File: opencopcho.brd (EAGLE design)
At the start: 51 parts, among them CON12 CON-4P-JST_GH-RA, CON13 CON-4P-JST_GH-RA, CON14 PINHEAD_1X02-2.54, CON15 PINHEAD_1X05-2.54-KEY, CON16 PINHEAD_1X05-2.54-KEY, CON17 PINHEAD_1X05-2.54-KEY, CON18 PINHEAD_1X05-2.54-KEY, CON5 CON-4P-JST_GH-RA, CON6 CON-4P-JST_GH-RA, CON7 PINHEAD_1X02-2.54, CON8 PINHEAD_2X04-PLS, CON9 PINHEAD_2X04-PLS, IC1 TPS54260, IC2 MCP2542WFD, IC6 MCP2542WFD

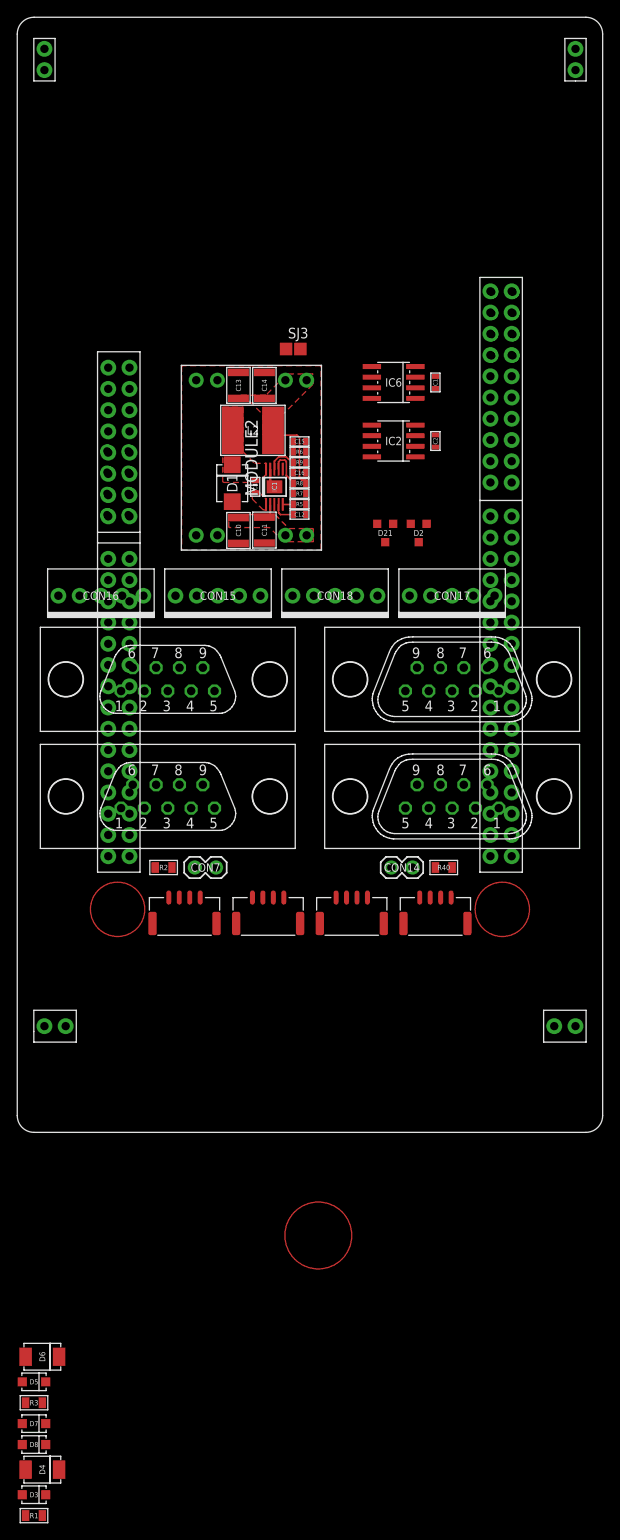
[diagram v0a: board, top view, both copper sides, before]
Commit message: updates
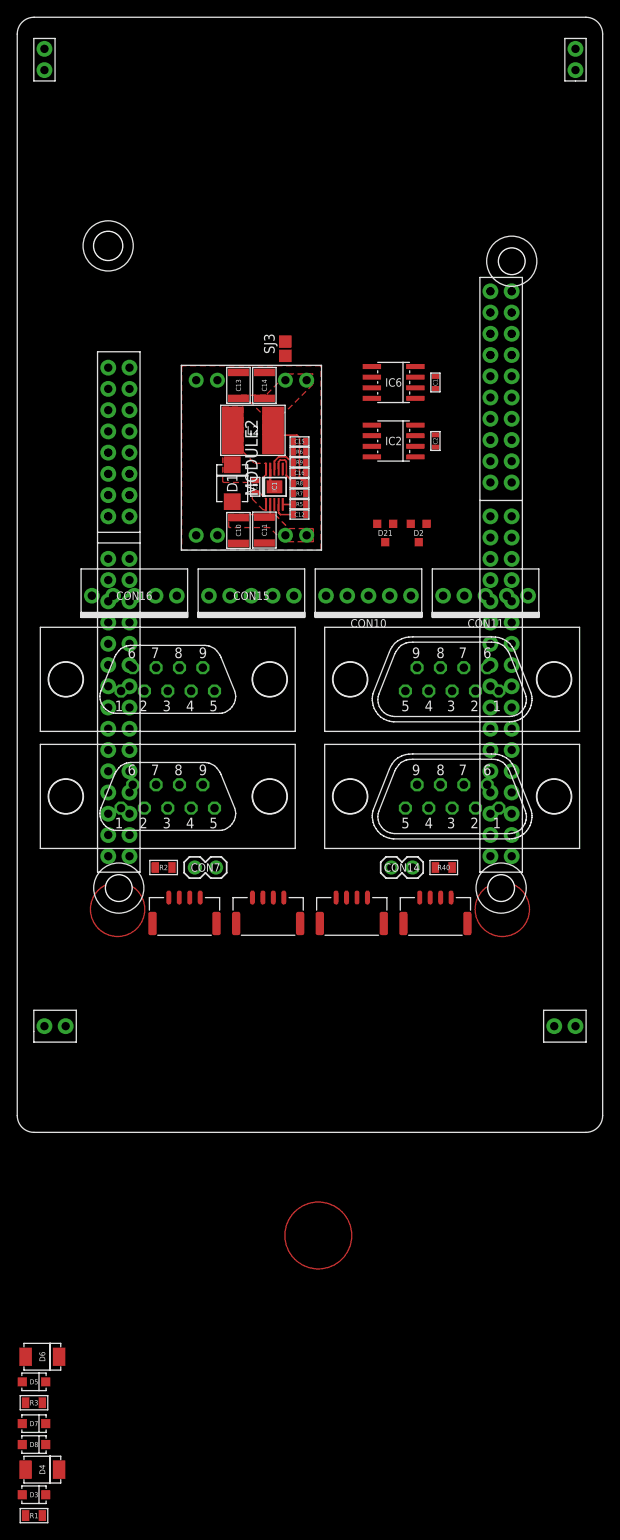
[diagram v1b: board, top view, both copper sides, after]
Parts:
- removed CON17, CON18: PINHEAD_1X05-2.54-KEY, pinhead:1X05-PTH-2.54-KEY
- added CON10, CON11: PINHEAD_1X05-2.54-KEY, pinhead:1X05-PTH-2.54-KEY
- moved CON15 4.00 mm to (-7.00, -2.50)
- moved CON16 4.00 mm to (-21.0, -2.50)
- moved SJ3 0.95 mm to (-2.95, 27.0), turned to 90 degrees
- moved CON9 0.25 mm to (-22.9, 10.8)
- moved CON8 0.17 mm to (22.9, 30.1)
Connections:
- net N$2 renamed VDD_24V
- removed net CAN_H: CON12.2, CON13.2, CON5.2, CON6.2, D2.1, D21.1, IC2.7, IC6.7, R2.1, R40.1
- removed net CAN_L: CON12.3, CON13.3, CON14.1, CON5.3, CON6.3, CON7.1, D2.2, D21.2, IC2.6, IC6.6
- new net CAN1_H: CON1.7, CON15.4, CON16.4, CON2.7, CON5.2, CON6.2, D2.1, IC2.7, R2.1
- new net CAN1_L: CON1.2, CON15.3, CON16.3, CON2.2, CON5.3, CON6.3, CON7.1, D2.2, IC2.6
- new net CAN1_SHIELD: CON15.2, CON16.2, CON2.5
- new net CAN1_VDD: CON1.9, CON15.5, CON16.5, CON2.9, R3.2
- new net CAN2_H: CON10.4, CON11.4, CON12.2, CON13.2, CON3.7, CON4.7, D21.1, IC6.7, R40.1
- new net CAN2_L: CON10.3, CON11.3, CON12.3, CON13.3, CON14.1, CON3.2, CON4.2, D21.2, IC6.6
- new net CAN2_SHIELD: CON10.2, CON11.2, CON3.5
- new net CAN2_VDD: CON10.5, CON11.5, CON3.9, R1.2
- net GND: now also CON1.6, CON10.1, CON11.1, CON15.1, CON16.1, CON2.6, CON3.6, CON4.6
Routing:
- added copper zone on layer 1, net N$6
- removed copper zone on layer 1, net VDD_5V
